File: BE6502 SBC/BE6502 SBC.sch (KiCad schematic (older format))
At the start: 61 parts, among them J1 Expansion, J2 CLOCK_SEL, J3 BARREL_JACK, J4 Control, M1 Mounting, M2 Mounting, M3 Mounting, M4 Mounting, SW1 RESET, SW2 MIDDLE, SW3 UP, SW4 DOWN, SW5 LEFT, SW6 RIGHT, U1 W65C02, U2 HM62256BLP-7, U3 28C256, U4 WD65C22, U5 74HC00, U6 RC1602A, U7 LM555, X1 1MHz

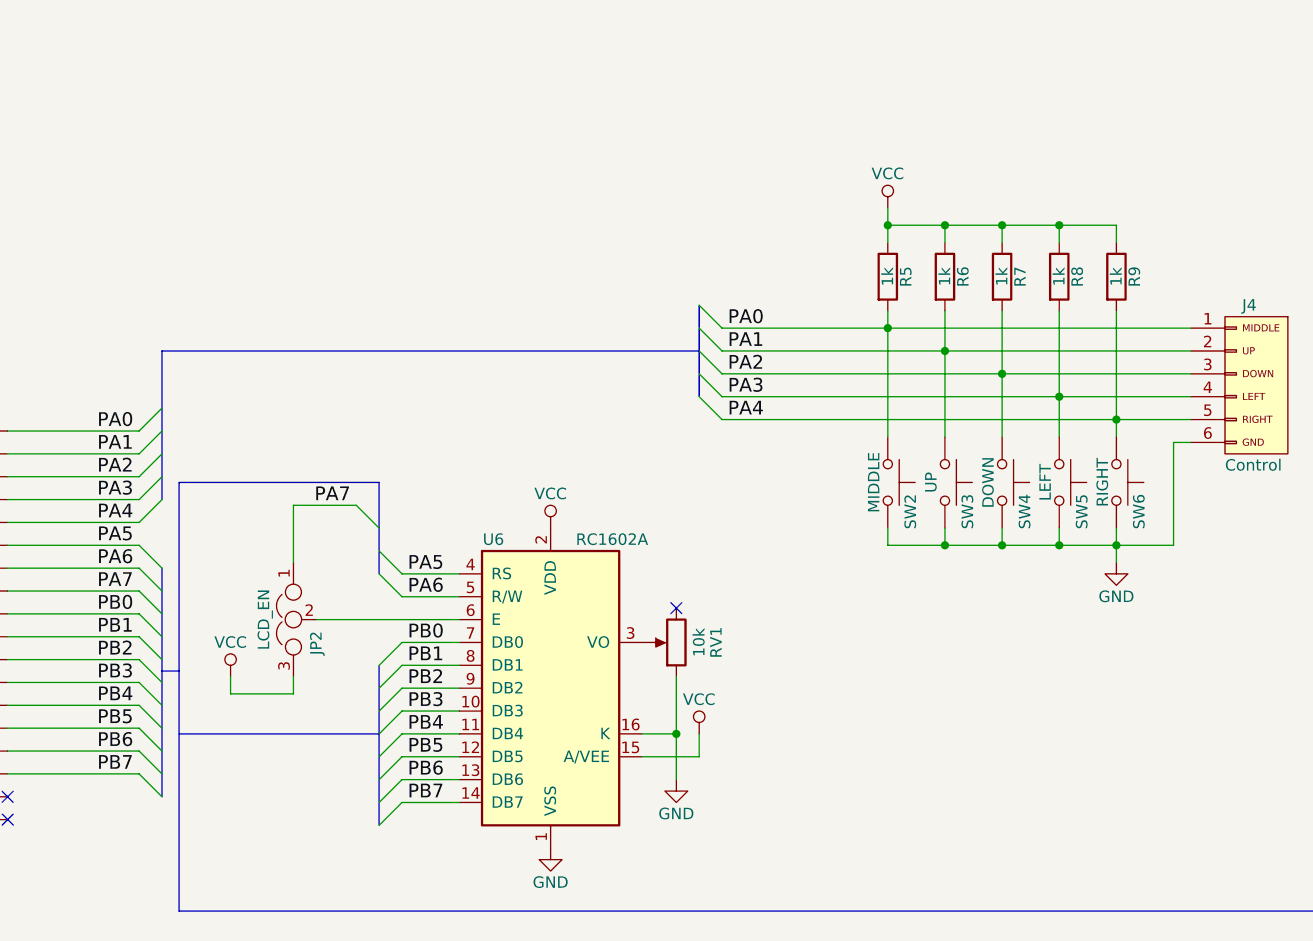
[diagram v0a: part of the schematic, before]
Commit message: make some basic changes
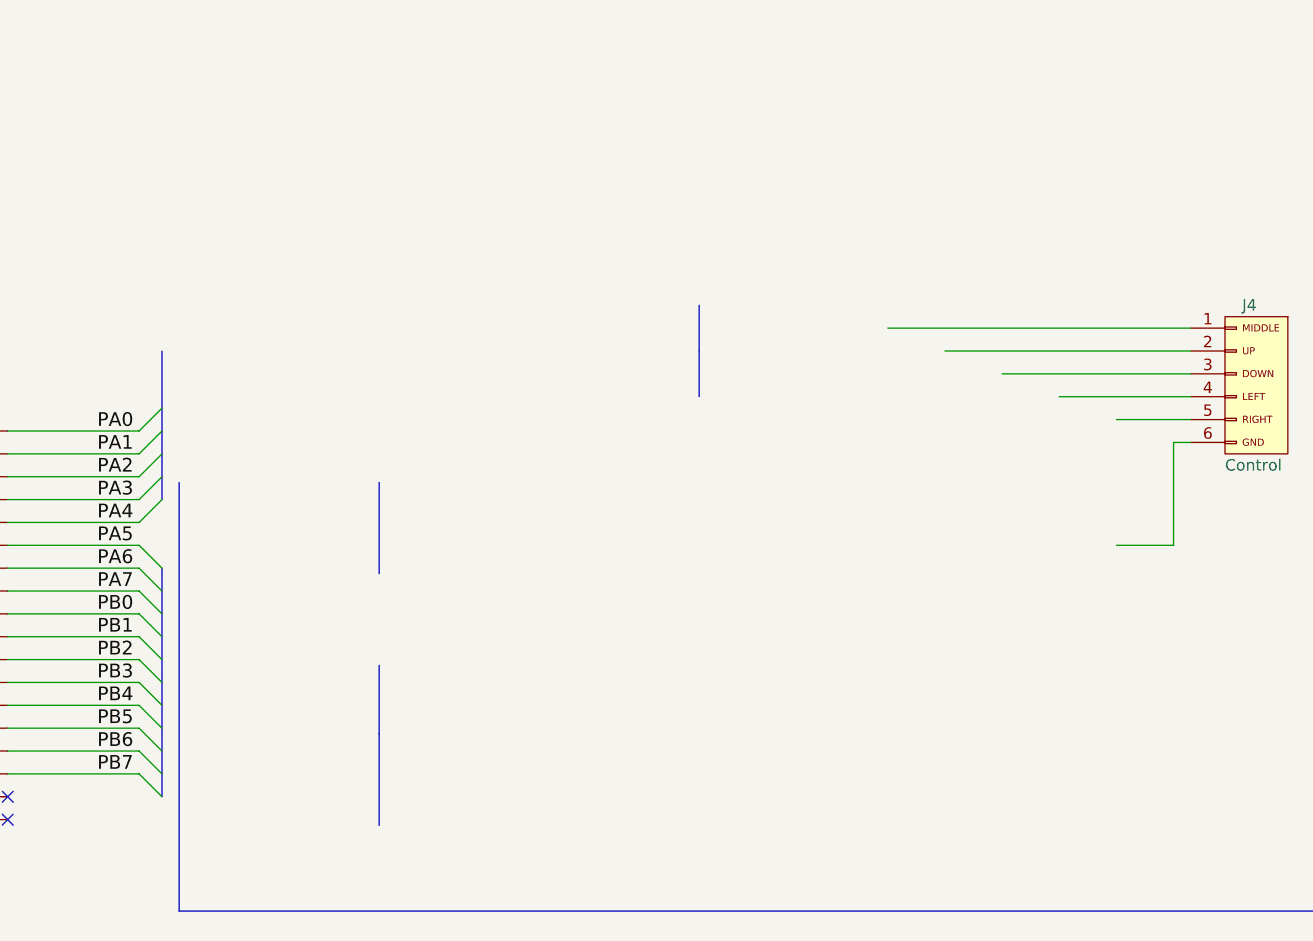
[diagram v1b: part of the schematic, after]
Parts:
- removed JP2: LCD_EN, Pin_Headers:Pin_Header_Straight_1x03_Pitch2.54mm, symbol Device:Jumper_NC_Dual
- removed R5, R6, R7, R8, R9: 1k, Resistors_THT:R_Axial_DIN0207_L6.3mm_D2.5mm_P10.16mm_Horizontal, symbol Device:R
- removed RV1: 10k, Potentiometers:Potentiometer_Trimmer_Bourns_3296W, symbol BE6502-SBC-rescue:POT
- removed SW2: MIDDLE, Buttons_Switches_THT:SW_PUSH_6mm, symbol switches:SW_Push
- removed SW3: UP, Buttons_Switches_THT:SW_PUSH_6mm, symbol switches:SW_Push
- removed SW4: DOWN, Buttons_Switches_THT:SW_PUSH_6mm, symbol switches:SW_Push
- removed SW5: LEFT, Buttons_Switches_THT:SW_PUSH_6mm, symbol switches:SW_Push
- removed SW6: RIGHT, Buttons_Switches_THT:SW_PUSH_6mm, symbol switches:SW_Push
- removed U6: RC1602A, lcd1602a:WC1602A, symbol 16x2_lcd:16x2_LCD
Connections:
- net GND: no longer J4.6 (GND)
- net PA0: no longer J4.1 (MIDDLE)
- net PA1: no longer J4.2 (UP)
- net PA2: no longer J4.3 (DOWN)
- net PA3: no longer J4.4 (LEFT)
- net PA4: no longer J4.5 (RIGHT)
- no-connect marks 12 -> 11

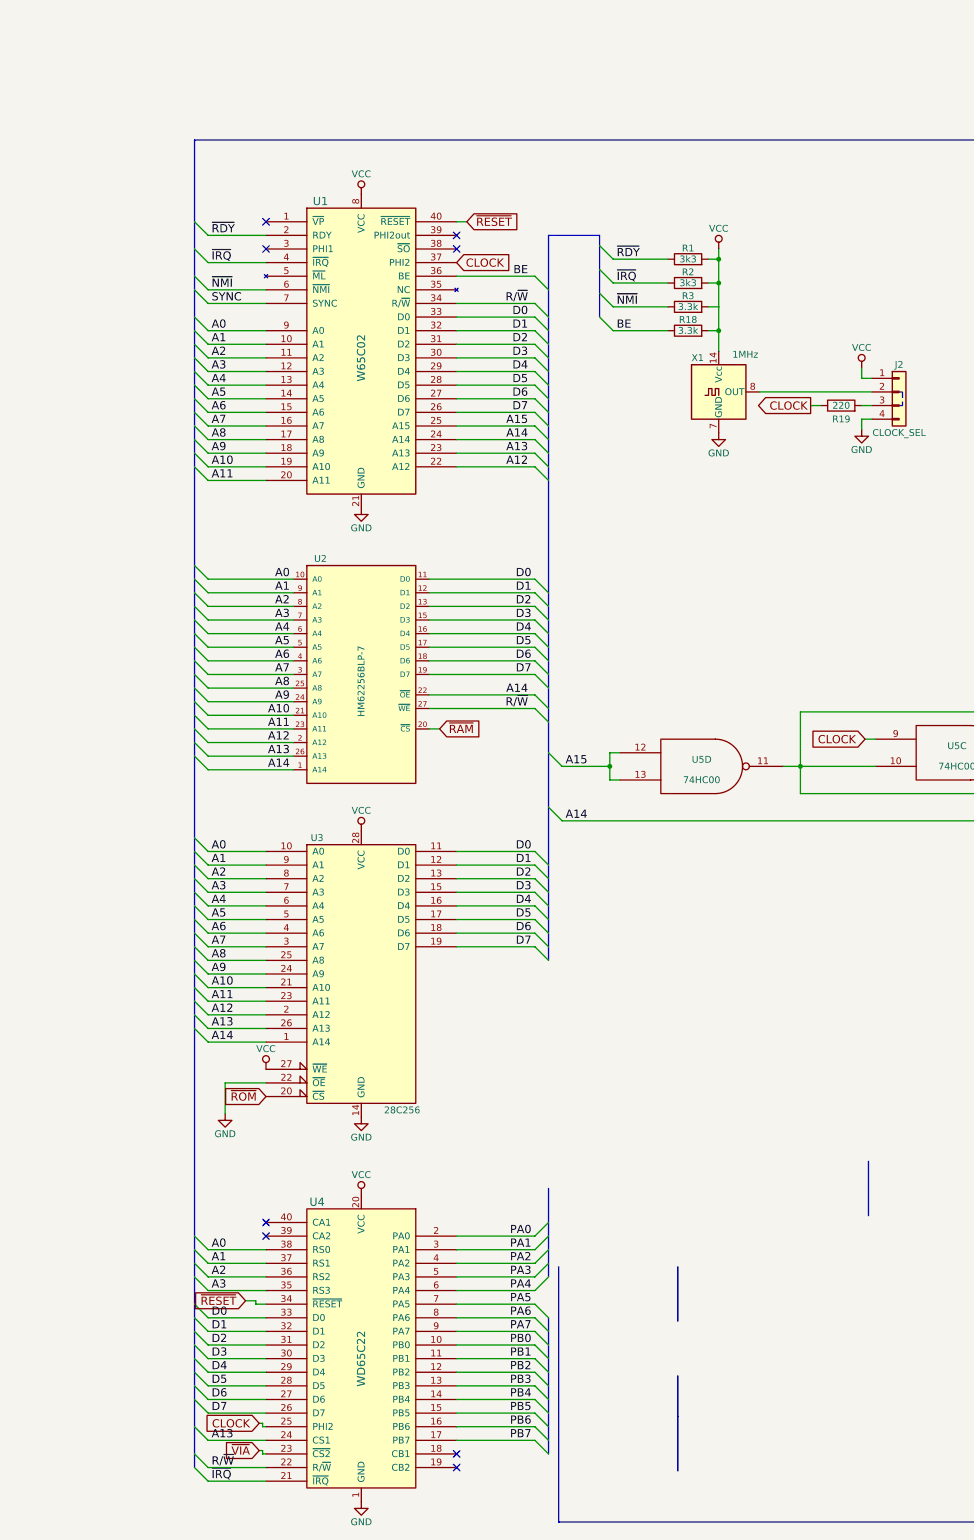
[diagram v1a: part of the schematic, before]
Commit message: Add a bunch of stuff
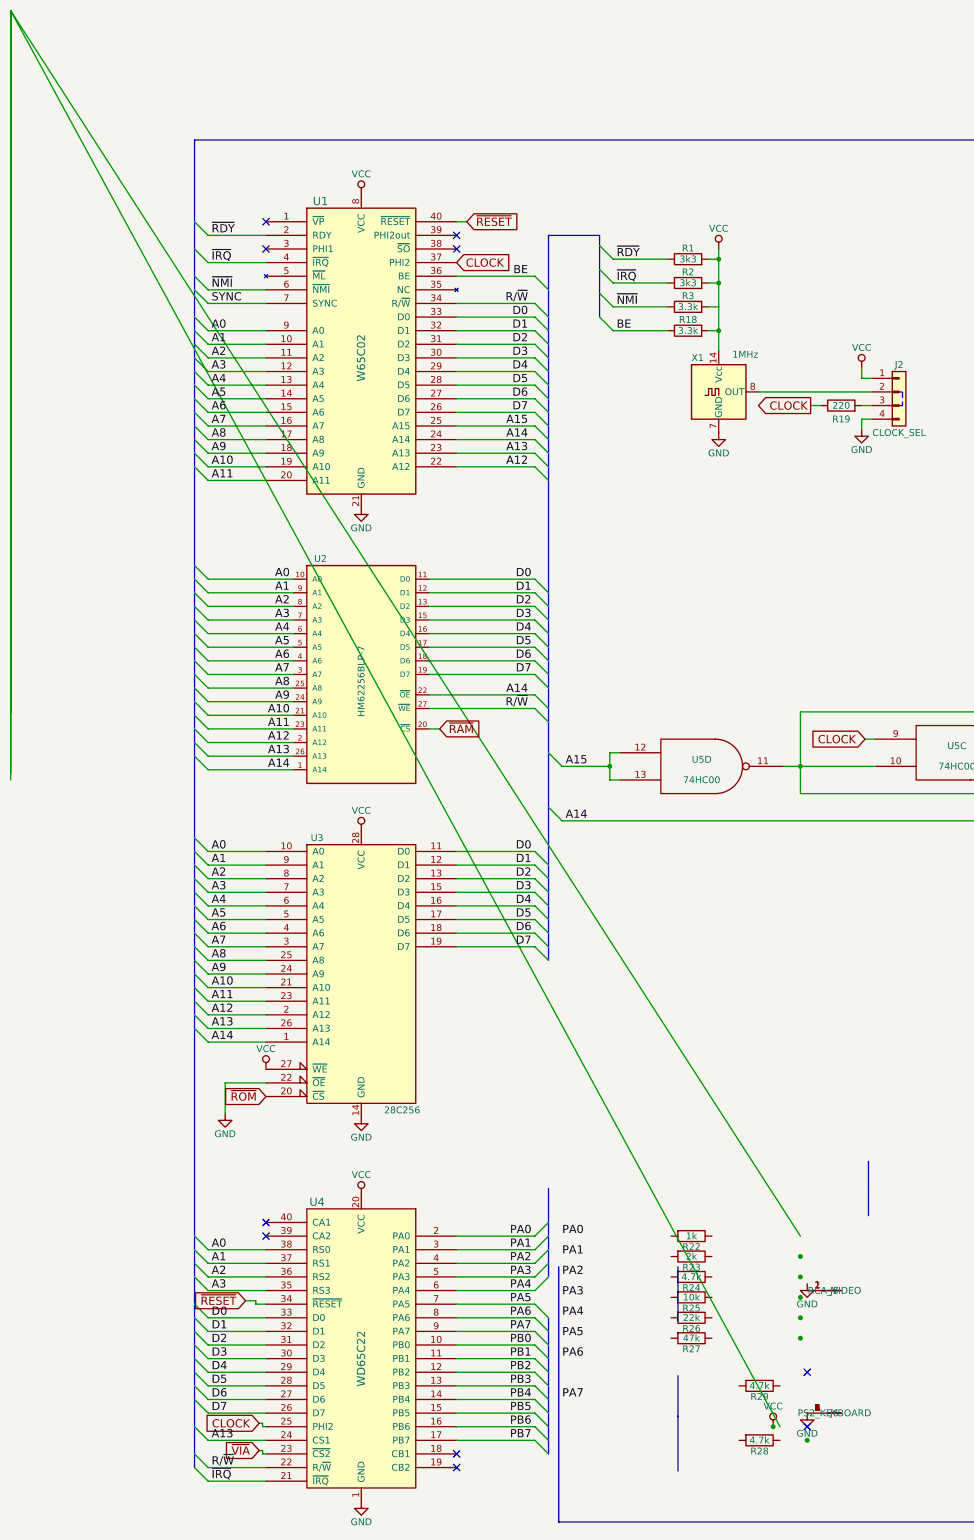
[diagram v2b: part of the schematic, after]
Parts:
- added J5: RCA_VIDEO, Connector:RCA_PJRA3x2_SMD, symbol conn:Conn_01x02
- added J6: PS2_KEYBOARD, Connector:PS2-6P, symbol conn:Conn_01x06
- added R22: 1k, Resistors_THT:R_Axial_DIN0207_L6.3mm_D2.5mm_P10.16mm_Horizontal, symbol Device:R
- added R23: 2k, Resistors_THT:R_Axial_DIN0207_L6.3mm_D2.5mm_P10.16mm_Horizontal, symbol Device:R
- added R24, R28, R29: 4.7k, Resistors_THT:R_Axial_DIN0207_L6.3mm_D2.5mm_P10.16mm_Horizontal, symbol Device:R
- added R25: 10k, Resistors_THT:R_Axial_DIN0207_L6.3mm_D2.5mm_P10.16mm_Horizontal, symbol Device:R
- added R26: 22k, Resistors_THT:R_Axial_DIN0207_L6.3mm_D2.5mm_P10.16mm_Horizontal, symbol Device:R
- added R27: 47k, Resistors_THT:R_Axial_DIN0207_L6.3mm_D2.5mm_P10.16mm_Horizontal, symbol Device:R
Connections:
- net GND: now also J6.1 (Pin_1), J6.2 (Pin_2), J6.3 (Pin_3), J6.4 (Pin_4), J6.5 (Pin_5), J6.6 (Pin_6)
- net PA0: now also R22.2
- net PA1: now also R23.2
- net PA2: now also R24.2
- net PA3: now also R25.2
- net PA4: now also R26.2
- net PA5: now also R27.2
- net VCC: now also R28.1, R29.1
- new net: R22.1, R23.1, R24.1, R25.1, R26.1, R27.1
- new net: J5.1 (Pin_1), J5.2 (Pin_2)
- no-connect marks 11 -> 13
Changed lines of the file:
@@
 NoConn ~ 3275 10700
 NoConn ~ 1875 1750
+# --- Composite Video RCA Output (VIA PA0-PA5 -> Resistor DAC) ---
+$Comp
+L Device:R R22
+U 1 1 9255357C
+P 5000 9000
+F 0 "R22" V 5080 9000 50  0000 C CNN
+F 1 "1k" V 5000 9000 50  0000 C CNN
+F 2 "Resistors_THT:R_Axial_DIN0207_L6.3mm_D2.5mm_P10.16mm_Horizontal" V 4930 9000 50  0001 C CNN
+F 3 "" H 5000 9000 50  0001 C CNN
+	1    5000 9000
+	0    1    1    0
+$EndComp
+$Comp
+L Device:R R23
+U 1 1 25E1AA8F
+P 5000 9150
+F 0 "R23" V 5080 9150 50  0000 C CNN
+F 1 "2k" V 5000 9150 50  0000 C CNN
+F 2 "Resistors_THT:R_Axial_DIN0207_L6.3mm_D2.5mm_P10.16mm_Horizontal" V 4930 9150 50  0001 C CNN
+F 3 "" H 5000 9150 50  0001 C CNN
+	1    5000 9150
+	0    1    1    0
+$EndComp
+$Comp
+L Device:R R24
+U 1 1 ADE8DC4B
+P 5000 9300
+F 0 "R24" V 5080 9300 50  0000 C CNN
+F 1 "4.7k" V 5000 9300 50  0000 C CNN
+F 2 "Resistors_THT:R_Axial_DIN0207_L6.3mm_D2.5mm_P10.16mm_Horizontal" V 4930 9300 50  0001 C CNN
+F 3 "" H 5000 9300 50  0001 C CNN
+	1    5000 9300
+	0    1    1    0
+$EndComp
+$Comp
+L Device:R R25
+U 1 1 668D00AB
+P 5000 9450
+F 0 "R25" V 5080 9450 50  0000 C CNN
+F 1 "10k" V 5000 9450 50  0000 C CNN
+F 2 "Resistors_THT:R_Axial_DIN0207_L6.3mm_D2.5mm_P10.16mm_Horizontal" V 4930 9450 50  0001 C CNN
+F 3 "" H 5000 9450 50  0001 C CNN
+	1    5000 9450
+	0    1    1    0
+$EndComp
+$Comp
+L Device:R R26
+U 1 1 0E26AE7C
+P 5000 9600
+F 0 "R26" V 5080 9600 50  0000 C CNN
+F 1 "22k" V 5000 9600 50  0000 C CNN
+F 2 "Resistors_THT:R_Axial_DIN0207_L6.3mm_D2.5mm_P10.16mm_Horizontal" V 4930 9600 50  0001 C CNN
+F 3 "" H 5000 9600 50  0001 C CNN
+	1    5000 9600
+	0    1    1    0
+$EndComp
+$Comp
+L Device:R R27
+U 1 1 FA9F5F78
+P 5000 9750
+F 0 "R27" V 5080 9750 50  0000 C CNN
+F 1 "47k" V 5000 9750 50  0000 C CNN
+F 2 "Resistors_THT:R_Axial_DIN0207_L6.3mm_D2.5mm_P10.16mm_Horizontal" V 4930 9750 50  0001 C CNN
+F 3 "" H 5000 9750 50  0001 C CNN
+	1    5000 9750
+	0    1    1    0
+$EndComp
+$Comp
+L conn:Conn_01x02 J5
+U 1 1 B4B321D2
+P 6050 9400
+F 0 "J5" H 6050 9625 50  0000 C CNN
+F 1 "RCA_VIDEO" H 6050 9125 50  0000 C CNN
+F 2 "Connector:RCA_PJRA3x2_SMD" H 6050 9400 50  0001 C CNN
+F 3 "" H 6050 9400 50  0001 C CNN
+	1    6050 9400
+	1    0    0    0
+$EndComp
+$Comp
+L power:GND #PWR032
+U 1 1 ACA60869
+P 5850 9350
+F 0 "#PWR032" H 5850 9100 50  0001 C CNN
+F 1 "GND" H 5850 9200 50  0000 C CNN
+F 2 "" H 5850 9350 50  0001 C CNN
+F 3 "" H 5850 9350 50  0001 C CNN
+	1    5850 9350
+	1    0    0    -1
+$EndComp
+Text Label 4050 9000 0    60   ~ 0
+PA0
+Text Label 4050 9150 0    60   ~ 0
+PA1
+Text Label 4050 9300 0    60   ~ 0
+PA2
+Text Label 4050 9450 0    60   ~ 0
+PA3
+Text Label 4050 9600 0    60   ~ 0
+PA4
+Text Label 4050 9750 0    60   ~ 0
+PA5
+Wire Wire Line 4050 9000 4850 9000
+Wire Wire Line 4050 9150 4850 9150
+Wire Wire Line 4050 9300 4850 9300
+Wire Wire Line 4050 9450 4850 9450
+Wire Wire Line 4050 9600 4850 9600
+Wire Wire Line 4050 9750 4850 9750
+Wire Wire Line 5150 9000 5800 9000
+Wire Wire Line 5150 9150 5800 9150
+Wire Wire Line 5150 9300 5800 9300
+Wire Wire Line 5150 9450 5800 9450
+Wire Wire Line 5150 9600 5800 9600
+Wire Wire Line 5150 9750 5800 9750
+Wire Wire Line 5800 9000 5800 9750
+Connection ~ 5800 9000
+Connection ~ 5800 9150
+Connection ~ 5800 9300
+Connection ~ 5800 9450
+Connection ~ 5800 9600
+Connection ~ 5800 9750
+Wire Wire Line 5800 9450 5850 9450
+# --- PS/2 Keyboard Port (VIA PA6=DATA, PA7=CLOCK -> mini-DIN) ---
+$Comp
+L conn:Conn_01x06 J6
+U 1 1 3005B9C2
+P 6050 10300
+F 0 "J6" H 6050 10600 50  0000 C CNN
+F 1 "PS2_KEYBOARD" H 6050 9975 50  0000 C CNN
+F 2 "Connector:PS2-6P" H 6050 10300 50  0001 C CNN
+F 3 "" H 6050 10300 50  0001 C CNN
+	1    6050 10300
+	1    0    0    0
+$EndComp
+$Comp
+L Device:R R28
+U 1 1 773A6297
+P 5500 10500
+F 0 "R28" V 5580 10500 50  0000 C CNN
+F 1 "4.7k" V 5500 10500 50  0000 C CNN
+F 2 "Resistors_THT:R_Axial_DIN0207_L6.3mm_D2.5mm_P10.16mm_Horizontal" V 5430 10500 50  0001 C CNN
+F 3 "" H 5500 10500 50  0001 C CNN
+	1    5500 10500
+	0    1    1    0
+$EndComp
+$Comp
+L Device:R R29
+U 1 1 E0A8B335
+P 5500 10100
+F 0 "R29" V 5580 10100 50  0000 C CNN
+F 1 "4.7k" V 5500 10100 50  0000 C CNN
+F 2 "Resistors_THT:R_Axial_DIN0207_L6.3mm_D2.5mm_P10.16mm_Horizontal" V 5430 10100 50  0001 C CNN
+F 3 "" H 5500 10100 50  0001 C CNN
+	1    5500 10100
+	0    1    1    0
+$EndComp
+$Comp
+L power:VCC #PWR033
+U 1 1 9CEDBA49
+P 5600 10400
+F 0 "#PWR033" H 5600 10250 50  0001 C CNN
+F 1 "VCC" H 5600 10550 50  0000 C CNN
+F 2 "" H 5600 10400 50  0001 C CNN
+F 3 "" H 5600 10400 50  0001 C CNN
+	1    5600 10400
+	1    0    0    -1
+$EndComp
+$Comp
+L power:GND #PWR034
+U 1 1 290EDEB8
+P 5850 10300
+F 0 "#PWR034" H 5850 10050 50  0001 C CNN
+F 1 "GND" H 5850 10150 50  0000 C CNN
+F 2 "" H 5850 10300 50  0001 C CNN
+F 3 "" H 5850 10300 50  0001 C CNN
+	1    5850 10300
+	1    0    0    -1
+$EndComp
+Text Label 4050 9900 0    60   ~ 0
+PA6
+Text Label 4050 10200 0    60   ~ 0
+PA7
+Wire Wire Line 4050 9900 5000 9900
+Wire Wire Line 4050 10200 5050 10200
+Wire Wire Line 5000 9900 5000 10500
+Wire Wire Line 5050 10200 5050 10100
+Wire Wire Line 5000 10500 5850 10500
+Wire Wire Line 5050 10100 5850 10100
+Wire Wire Line 5600 10400 5650 10400
+Wire Wire Line 5650 10400 5650 10500
+Wire Wire Line 5650 10400 5650 10100
+Wire Wire Line 5600 10400 5600 10200
+Wire Wire Line 5600 10200 5850 10200
+Connection ~ 5650 10400
+Connection ~ 5600 10400
+Connection ~ 5850 10500
+NoConn ~ 5850 10400
+NoConn ~ 5850 10000
 Text Notes 11825 10250 0    60   ~ 0
 This is a PCB version of the 6502 computer featured in Ben Eaters "Build a 6502\ncomputer" series of videos. Based on the schematics on his website, at the \nrelease of part 7 of his series.
